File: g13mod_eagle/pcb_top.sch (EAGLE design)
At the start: 4 parts

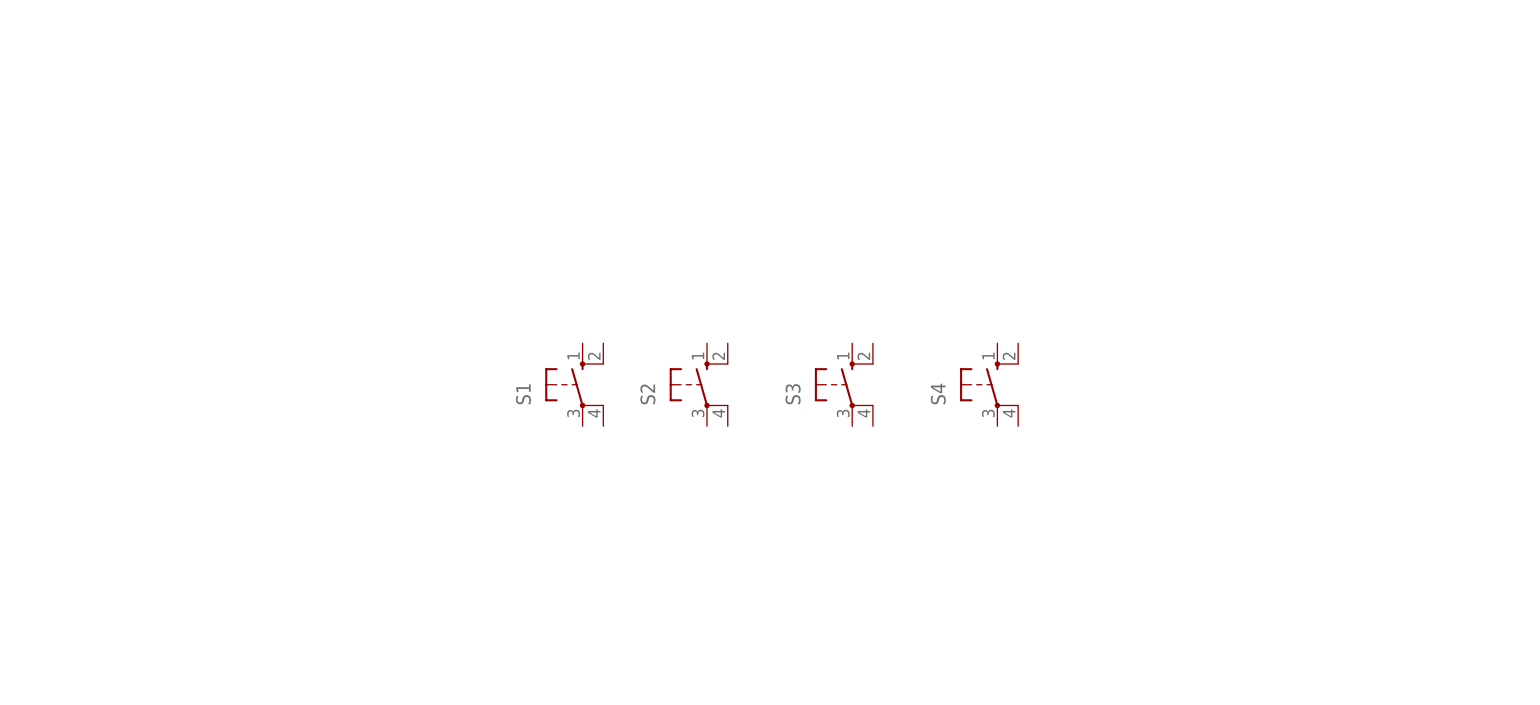
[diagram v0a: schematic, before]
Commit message: wiring
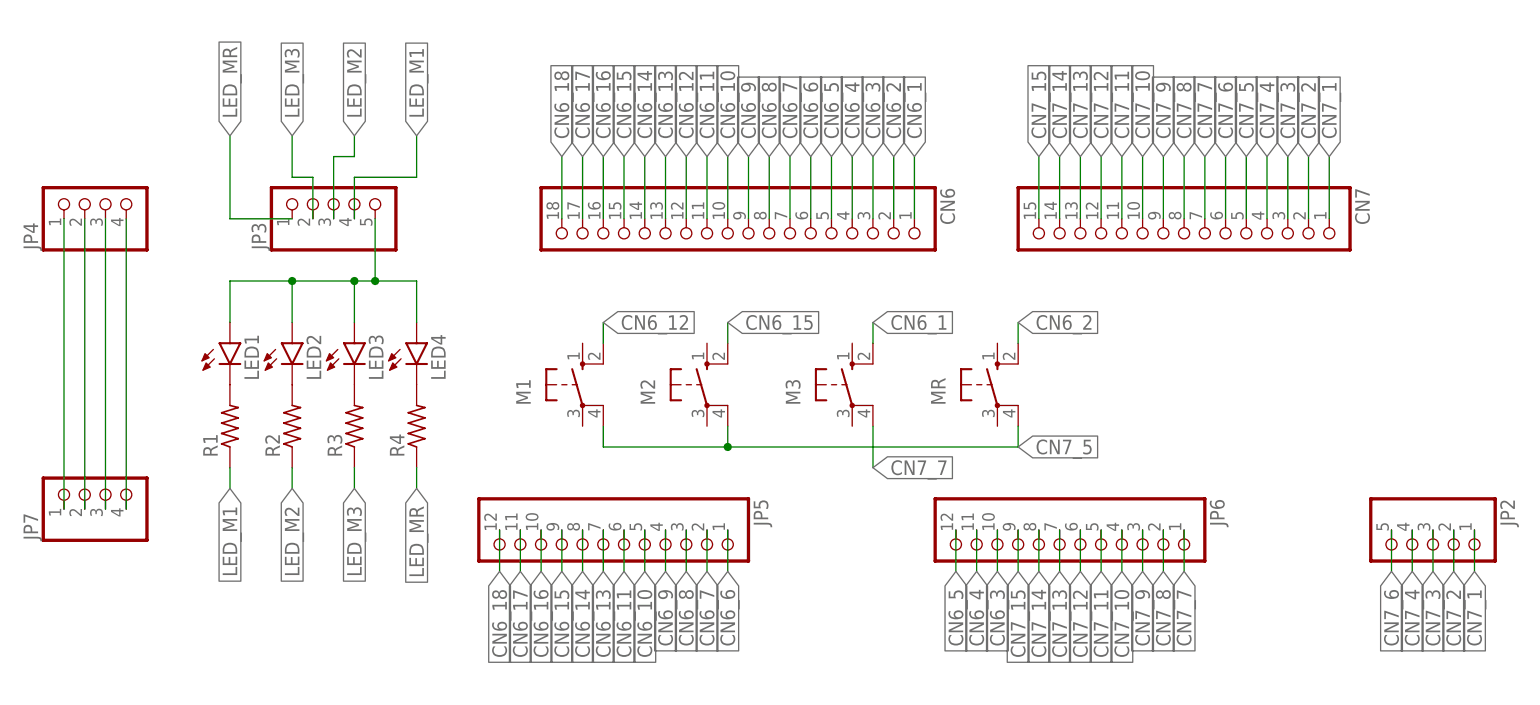
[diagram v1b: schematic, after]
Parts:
- added CN6: (no value), pinhead-half-pitch:THROUHOLE18
- added CN7: (no value), pinhead-half-pitch:THROUHOLE15
- added JP2, JP3: (no value), pinhead-half-pitch:THROUHOLE05
- added JP4, JP7: (no value), pinhead-half-pitch:THROUHOLE04
- added JP5, JP6: (no value), pinhead-half-pitch:THROUHOLE12
- added LED1, LED2, LED3, LED4: (no value), led:LEDCHIPLED_1206
- added R1, R2, R3, R4: (no value), rcl:R-US_R0603
- renumbered S1 to M1, S2 to M2, S3 to M3, S4 to MR
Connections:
- new net CN6_1: CN6.1, M3.S1
- new net CN6_10: CN6.10, JP5.5
- new net CN6_11: CN6.11, JP5.6
- new net CN6_12: CN6.12, M1.S1
- new net CN6_13: CN6.13, JP5.7
- new net CN6_14: CN6.14, JP5.8
- new net CN6_15: CN6.15, JP5.9, M2.S1
- new net CN6_16: CN6.16, JP5.10
- new net CN6_17: CN6.17, JP5.11
- new net CN6_18: CN6.18, JP5.12
- new net CN6_2: CN6.2, MR.S1
- new net CN6_3: CN6.3, JP6.10
- new net CN6_4: CN6.4, JP6.11
- new net CN6_5: CN6.5, JP6.12
- new net CN6_6: CN6.6, JP5.1
- new net CN6_7: CN6.7, JP5.2
- new net CN6_8: CN6.8, JP5.3
- new net CN6_9: CN6.9, JP5.4
- new net CN7_1: CN7.1, JP2.1
- new net CN7_10: CN7.10, JP6.4
- new net CN7_11: CN7.11, JP6.5
- new net CN7_12: CN7.12, JP6.6
- new net CN7_13: CN7.13, JP6.7
- new net CN7_14: CN7.14, JP6.8
- new net CN7_15: CN7.15, JP6.9
- new net CN7_2: CN7.2, JP2.2
- new net CN7_3: CN7.3, JP2.3
- new net CN7_4: CN7.4, JP2.4
- new net CN7_5: CN7.5, M1.P1, M2.P1, MR.P1
- new net CN7_6: CN7.6, JP2.5
- new net CN7_7: CN7.7, JP6.1, M3.P1
- new net CN7_8: CN7.8, JP6.2
- new net CN7_9: CN7.9, JP6.3
- new net LED_M1: JP3.4, R1.1
- new net LED_M2: JP3.3, R2.1
- new net LED_M3: JP3.2, R3.1
- new net LED_MR: JP3.1, R4.1
- new net N$1: JP4.1, JP7.1
- new net N$2: JP4.2, JP7.2
- new net N$3: JP4.3, JP7.3
- new net N$4: JP4.4, JP7.4
- new net N$5: JP3.5, LED1.A, LED2.A, LED3.A, LED4.A
- new net N$6: LED1.C, R1.2
- new net N$7: LED2.C, R2.2
- new net N$8: LED3.C, R3.2
- new net N$9: LED4.C, R4.2
